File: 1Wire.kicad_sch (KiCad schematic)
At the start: 14 parts, among them J12 Conn_01x03_Male, J13 Conn_01x02, J2 Conn_01x03, U1 ESP-01v090, U3 DS18B20, U4 HT73xx-1-SOT89

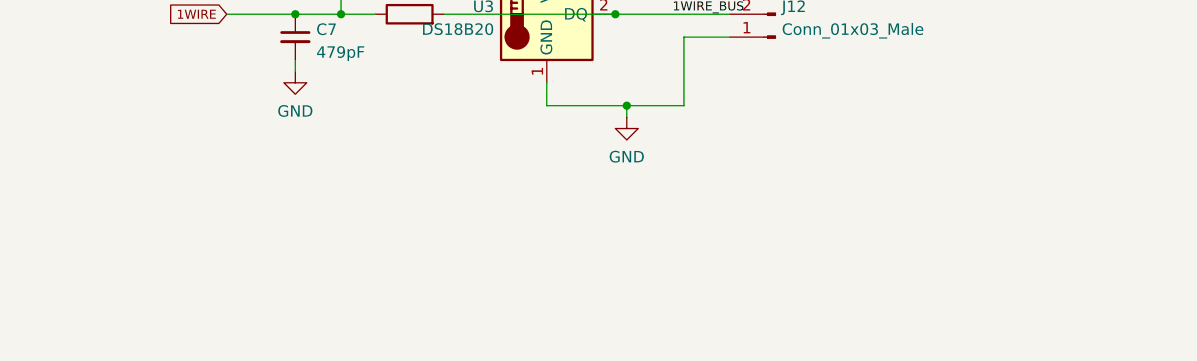
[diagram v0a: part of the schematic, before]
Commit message: Add files via upload
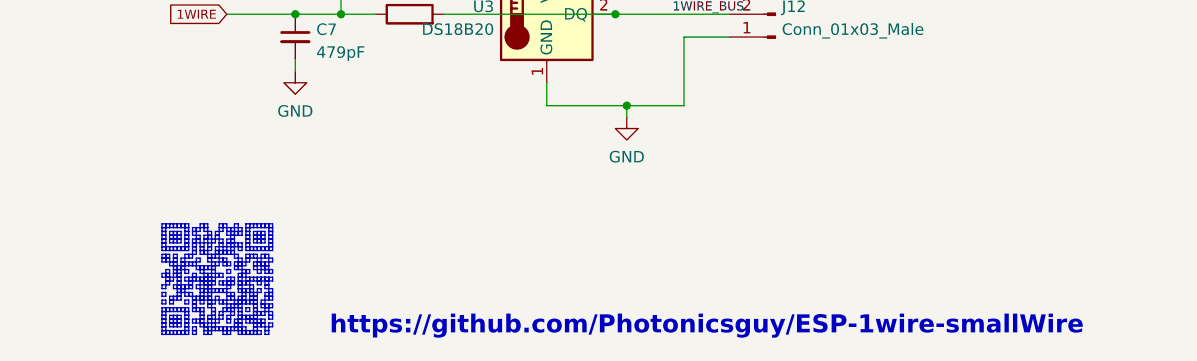
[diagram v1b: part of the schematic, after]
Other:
- note added: "https://github.com/Photonicsguy/ESP-1wire-smallWire"
